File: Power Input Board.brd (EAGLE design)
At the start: 136.7 x 125.3 mm, 19 parts, among them Q1 SPB80P06P

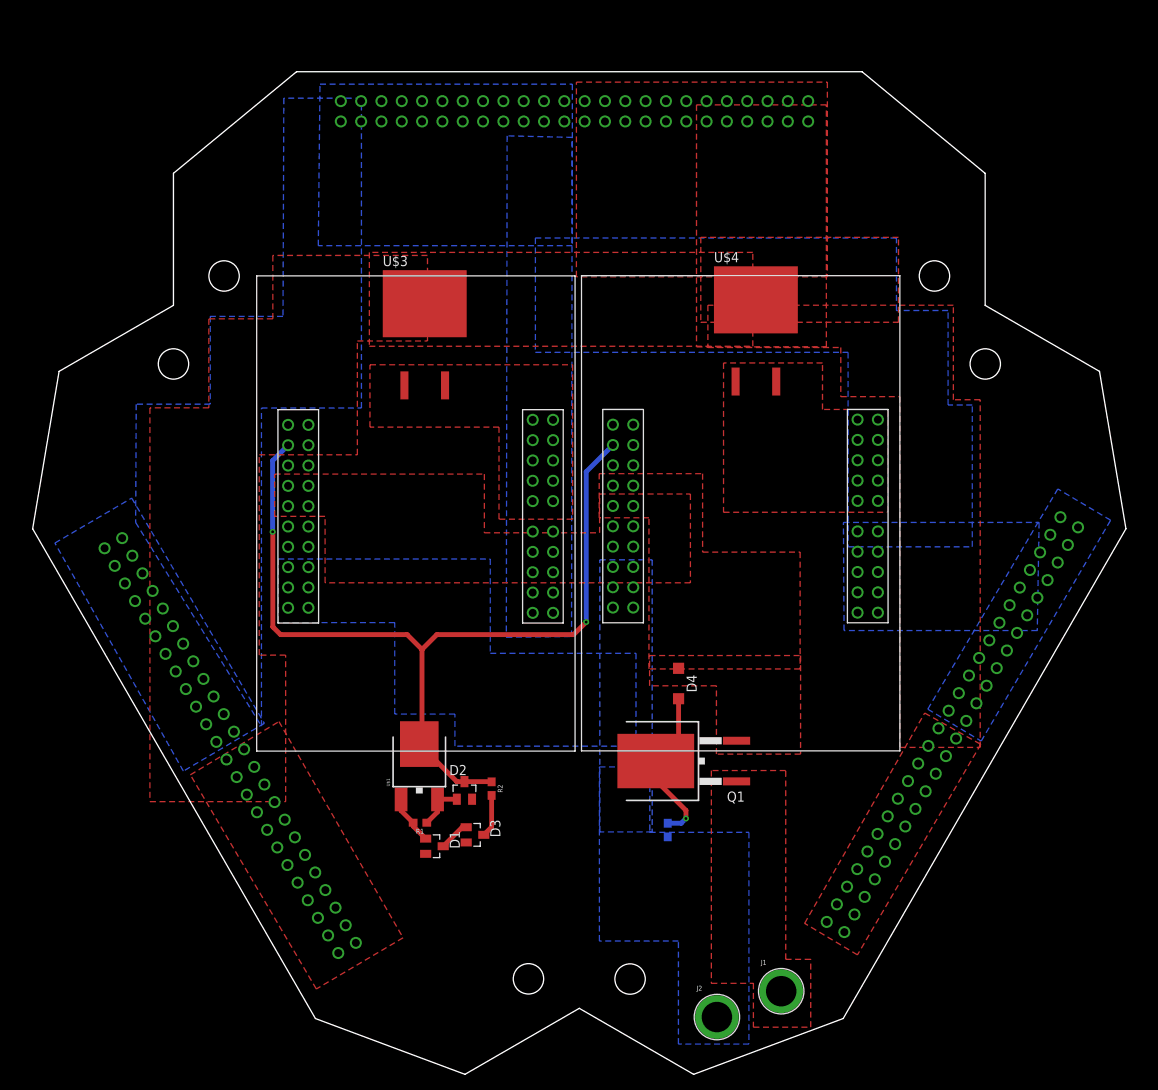
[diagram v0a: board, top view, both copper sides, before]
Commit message: rerouted
rerouted everything
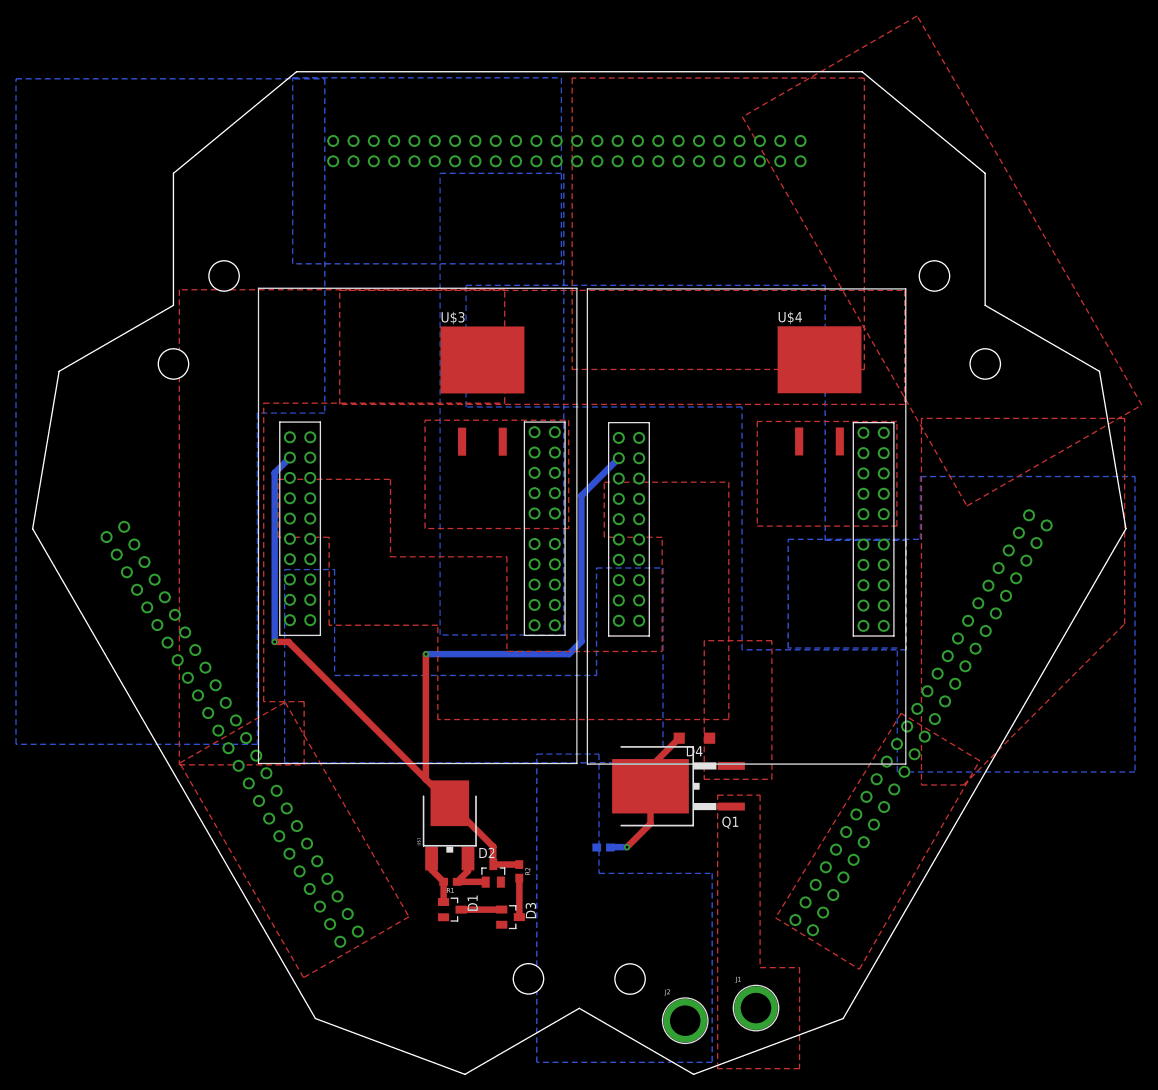
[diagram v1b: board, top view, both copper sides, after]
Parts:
- removed U$8, U$9: PDB_PCB_CONNEC, PDB_PCB_connectors:PDB_PCB
- U$7: device PDB_PCB_connectors:PDB_PCB -> PDB_PCB_connectors:PDB_PCB_2
- moved U$7 50.1 mm to (0.00, 0.00), turned to 0 degrees
- moved D3 11.2 mm to (59.7, 19.7)
- moved D2 11.0 mm to (57.6, 25.1)
- moved U$4 10.9 mm to (93.1, 85.1)
- moved R2 10.9 mm to (60.8, 25.4)
- moved U$3 10.1 mm to (51.0, 85.1)
- moved R3 8.32 mm to (71.4, 28.4), turned to 180 degrees
- moved R1 8.32 mm to (52.2, 24.1)
- moved U$1 8.32 mm to (52.1, 32.3)
- moved D1 8.23 mm to (52.5, 20.6)
- moved D4 7.11 mm to (82.7, 42.0), turned to 180 degrees
- moved J2 3.99 mm to (81.6, 6.70)
- moved J1 3.79 mm to (90.4, 8.28)
- moved Q1 3.22 mm to (80.7, 36.0)
- moved U$6 1.81 mm to (69.3, 98.2)
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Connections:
- net +12V: now also U$7.+12V25, U$7.+12V26, U$7.+12V27, U$7.+12V28, U$7.+12V29, U$7.+12V30, U$7.+12V31, U$7.+12V32, U$7.+12V33, U$7.+12V34, U$7.+12V35, U$7.+12V36, U$7.+12V37, U$7.+12V38, U$7.+12V39, U$7.+12V40, U$7.+12V41, U$7.+12V42, U$7.+12V43, U$7.+12V44, U$7.+12V45, U$7.+12V46, U$7.+12V47, U$7.+12V48, U$7.+12V49, U$7.+12V50, U$7.+12V51, U$7.+12V52, U$7.+12V53, U$7.+12V54, U$7.+12V55, U$7.+12V56, U$7.+12V57, U$7.+12V58, U$7.+12V59, U$7.+12V60, U$7.+12V61, U$7.+12V62, U$7.+12V63, U$7.+12V64, U$7.+12V65, U$7.+12V66, U$7.+12V67, U$7.+12V68, U$7.+12V69, U$7.+12V70, U$7.+12V71, U$7.+12V72; no longer U$8.+12V1, U$8.+12V10, U$8.+12V11, U$8.+12V12, U$8.+12V13, U$8.+12V14, U$8.+12V15, U$8.+12V16, U$8.+12V17, U$8.+12V18, U$8.+12V19, U$8.+12V2, U$8.+12V20, U$8.+12V21, U$8.+12V22, U$8.+12V23, U$8.+12V24, U$8.+12V3, U$8.+12V4, U$8.+12V5, U$8.+12V6, U$8.+12V7, U$8.+12V8, U$8.+12V9, U$9.+12V1, U$9.+12V10, U$9.+12V11, U$9.+12V12, U$9.+12V13, U$9.+12V14, U$9.+12V15, U$9.+12V16, U$9.+12V17, U$9.+12V18, U$9.+12V19, U$9.+12V2, U$9.+12V20, U$9.+12V21, U$9.+12V22, U$9.+12V23, U$9.+12V24, U$9.+12V3, U$9.+12V4, U$9.+12V5, U$9.+12V6, U$9.+12V7, U$9.+12V8, U$9.+12V9
- net GND: now also U$7.GND1, U$7.GND25, U$7.GND26, U$7.GND27, U$7.GND28, U$7.GND29, U$7.GND30, U$7.GND31, U$7.GND32, U$7.GND33, U$7.GND34, U$7.GND35, U$7.GND36, U$7.GND37, U$7.GND38, U$7.GND39, U$7.GND40, U$7.GND41, U$7.GND42, U$7.GND43, U$7.GND44, U$7.GND45, U$7.GND46, U$7.GND47, U$7.GND48, U$7.GND49, U$7.GND50, U$7.GND51, U$7.GND52, U$7.GND53, U$7.GND54, U$7.GND55, U$7.GND56, U$7.GND57, U$7.GND58, U$7.GND59, U$7.GND60, U$7.GND61, U$7.GND62, U$7.GND63, U$7.GND64, U$7.GND65, U$7.GND66, U$7.GND67, U$7.GND68, U$7.GND69, U$7.GND70, U$7.GND71, U$7.GND72; no longer U$8.GND10, U$8.GND11, U$8.GND12, U$8.GND13, U$8.GND14, U$8.GND15, U$8.GND16, U$8.GND17, U$8.GND18, U$8.GND19, U$8.GND2, U$8.GND20, U$8.GND21, U$8.GND22, U$8.GND23, U$8.GND24, U$8.GND3, U$8.GND4, U$8.GND5, U$8.GND6, U$8.GND7, U$8.GND8, U$8.GND9, U$9.GND10, U$9.GND11, U$9.GND12, U$9.GND13, U$9.GND14, U$9.GND15, U$9.GND16, U$9.GND17, U$9.GND18, U$9.GND19, U$9.GND2, U$9.GND20, U$9.GND21, U$9.GND22, U$9.GND23, U$9.GND24, U$9.GND3, U$9.GND4, U$9.GND5, U$9.GND6, U$9.GND7, U$9.GND8, U$9.GND9
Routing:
- net ON/OFF: track 111.9 -> 127.8 mm
- net N$3: track 20.2 -> 18.4 mm
- net N$1: track 3.85 -> 5.08 mm
- net 3.3V: track 5.90 -> 7.08 mm
